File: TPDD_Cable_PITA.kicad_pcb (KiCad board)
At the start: 2 copper layers, 34.6 x 10.1 mm, 5 parts, among them J1 7 x wire pads, J2 DB25_Male, Q1 DTA114EKA, Q2 DTA114EKA, Q3 DTA114EKA

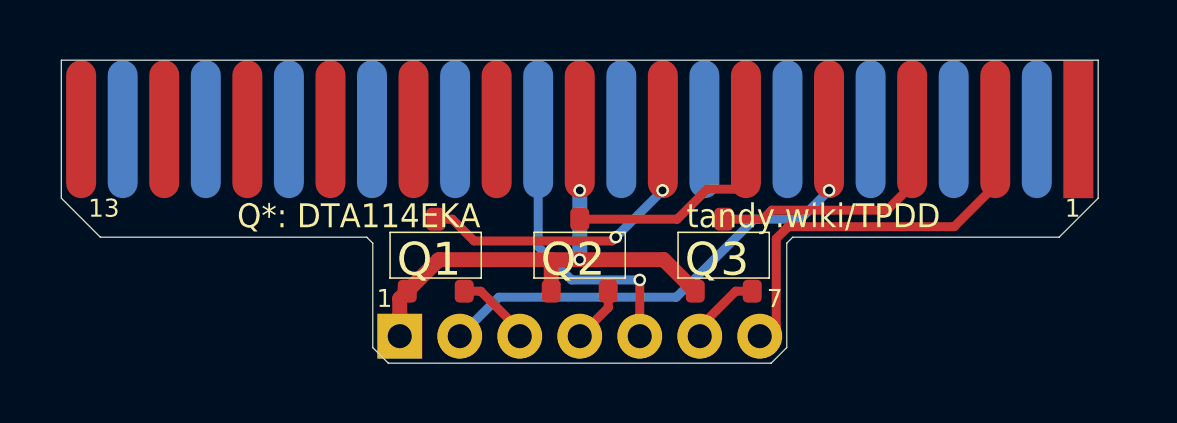
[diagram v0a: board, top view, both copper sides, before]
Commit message: pcbway limits, readme
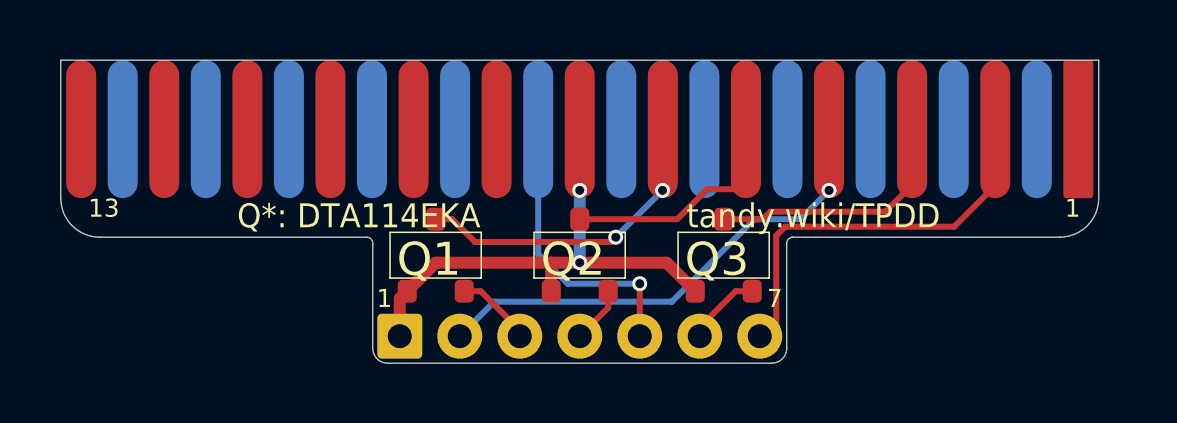
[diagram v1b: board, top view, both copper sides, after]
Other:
- net class Default: clearance 0.16 -> 0.2; trace_width 0.16 -> 0.2; via_dia 0.42 -> 0.5; via_drill 0.26 -> 0.3
- rule trace_clearance: 0.16 -> 0.2
- rule trace_min: 0.16 -> 0.2
- rule via_min_drill: 0.26 -> 0.3
- rule via_min_size: 0.42 -> 0.5
